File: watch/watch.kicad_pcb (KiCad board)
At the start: 4 copper layers, 38 x 38 mm, 91 parts, among them U1 STM32L071CBTx, Y1 3131M-32.768DTTLRRL

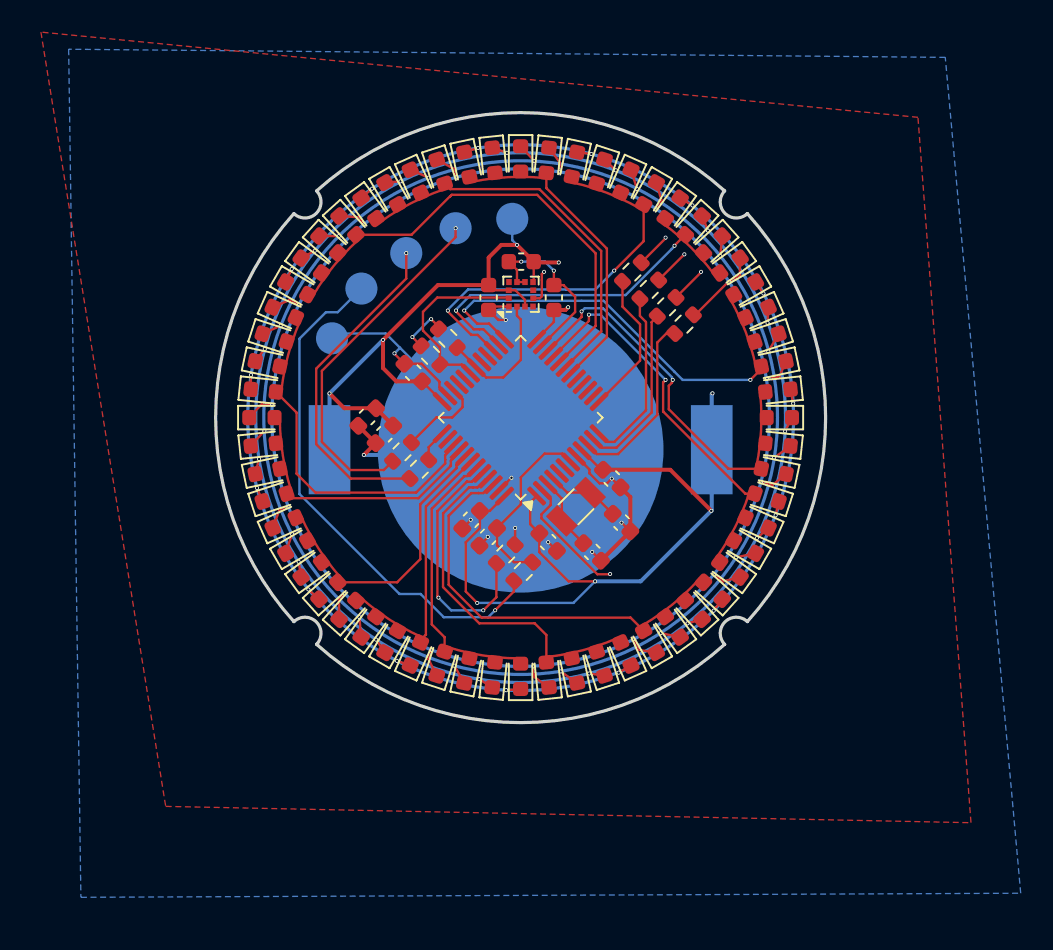
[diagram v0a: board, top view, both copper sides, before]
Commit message: V1.6 done?
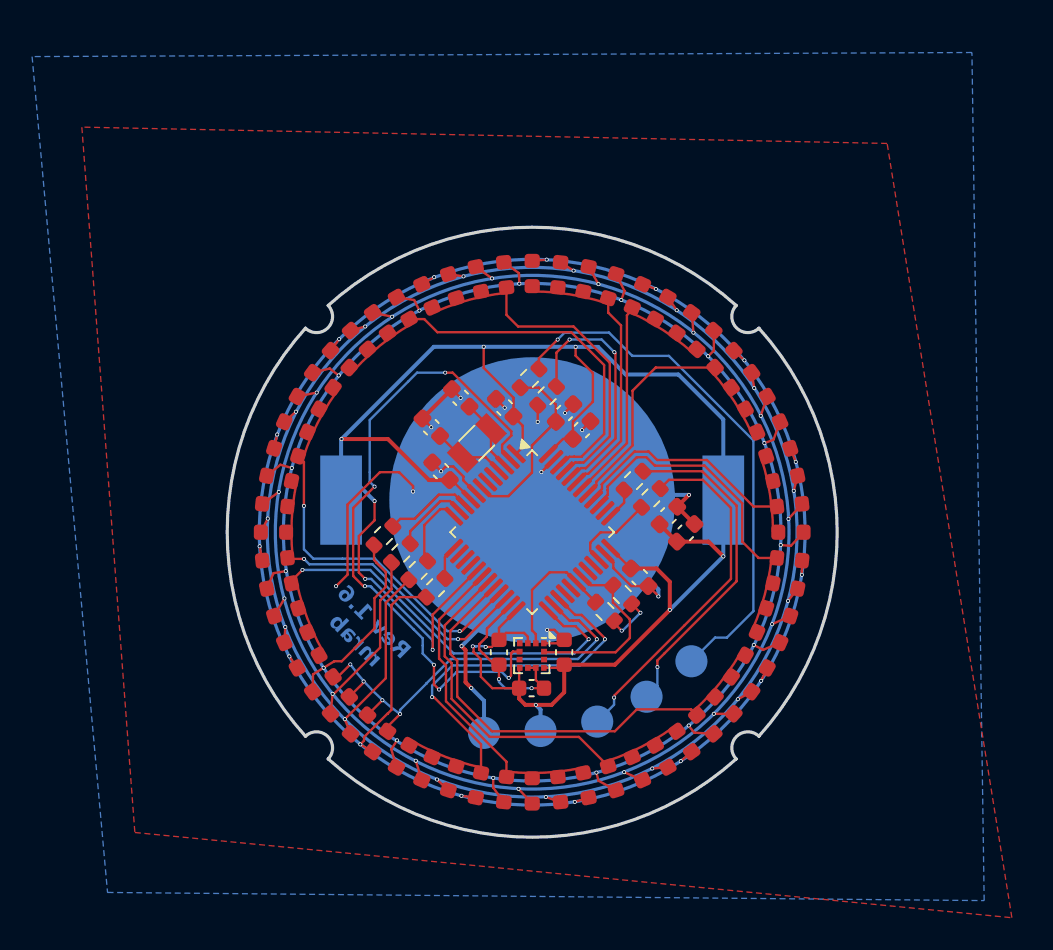
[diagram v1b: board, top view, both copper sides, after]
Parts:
- D1, D10, D11, D12, D13, D14, D15, D16, D17, D18, D19, D2, D20, D21, D22, D23, D24, D25, D26, D27, D28, D29, D3, D30, D31, D32, D33, D34, D35, D36, D37, D38, D39, D4, D40, D41, D42, D43, D44, D45, D46, D47, D48, D49, D5, D50, D51, D52, D53, D54, D55, D56, D57, D58, D59, D6, D60, D7, D8, D9: footprint LED_SMD:LED_0603_1608Metric -> LED_Without_Dot:0603
- R4, R5, R6, R7: value 100 -> 160
- U2: value ~ -> BOSCH BMA400
- moved D3 39.4 mm to (52.4, 73.2), turned to 96 degrees
- moved D2 39.4 mm to (50.7, 73.3), turned to 90 degrees
- moved D4 39.4 mm to (54.1, 72.9), turned to 102 degrees
- moved D1 39.3 mm to (49.0, 73.2), turned to 84 degrees
- moved D5 39.3 mm to (55.7, 72.5), turned to 108 degrees
- moved D60 39.1 mm to (47.4, 72.9), turned to 78 degrees
- moved D6 39.1 mm to (57.3, 71.9), turned to 114 degrees
- moved D59 38.9 mm to (45.7, 72.5), turned to 72 degrees
- moved D7 38.9 mm to (58.8, 71.1), turned to 120 degrees
- moved D58 38.6 mm to (44.2, 71.9), turned to 66 degrees
- moved D8 38.6 mm to (60.2, 70.2), turned to 126 degrees
- moved D57 38.3 mm to (42.7, 71.1), turned to 60 degrees
- moved D9 38.3 mm to (61.5, 69.1), turned to 132 degrees
- moved D56 37.9 mm to (41.2, 70.2), turned to 54 degrees
- moved D10 37.9 mm to (62.7, 67.9), turned to 138 degrees
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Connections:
- U1 pad 17: unconnected-(U1-PA7-Pad17) -> VDD
- U2 pad 10: unconnected-(U2-NC-Pad10) -> VDD
- U2 pad 11: VDD -> unconnected-(U2-PS-Pad11)
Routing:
- net IMU_WAKEUP_INTERRUPT: track 30.6 -> 40.8 mm, vias 2 -> 6
- net VDD: track 123.9 -> 133.7 mm, vias 11 -> 13
- net Net-(D12-K): track 18.3 -> 25.3 mm, vias 16 -> 15
- net LED_SINK_ROW3_GPIO: track 9.00 -> 2.11 mm
- net Net-(D1-K): track 30.1 -> 36.9 mm
- net LED_SINK_ROW2_GPIO: track 11.1 -> 4.75 mm
- net LED_SINK_ROW1_GPIO: track 10.9 -> 4.86 mm
- net Net-(D11-K): track 18.9 -> 24.9 mm, vias 16 -> 15
- net Net-(D10-K): track 22.6 -> 28.5 mm, vias 16 -> 15
- net LED_SINK_ROW0_GPIO: track 11.4 -> 5.58 mm
- net GND: track 76.6 -> 82.1 mm, vias 13 -> 17
- net LED_SOURCE_COLUMN11: track 20.2 -> 16.7 mm
- net LED_SOURCE_COLUMN13: track 19.9 -> 23.4 mm, vias 2 -> 5
- net LED_SOURCE_COLUMN14: track 20.2 -> 22.7 mm
- net LED_SOURCE_COLUMN4: track 12.3 -> 14.3 mm
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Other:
- copper layers 4 -> 2
- board text added: "GND"
- board text added: "JLCJLCJLCJLC"
- board text added: "NRST"
- board text added: "Rev 1.6 mrab"
- board text added: "SWCLK"
- board text added: "SWDIO"
- board text added: "VDD"
